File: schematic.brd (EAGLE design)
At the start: 72 x 26 mm, 27 parts, among them IC1 MEGA8-AI

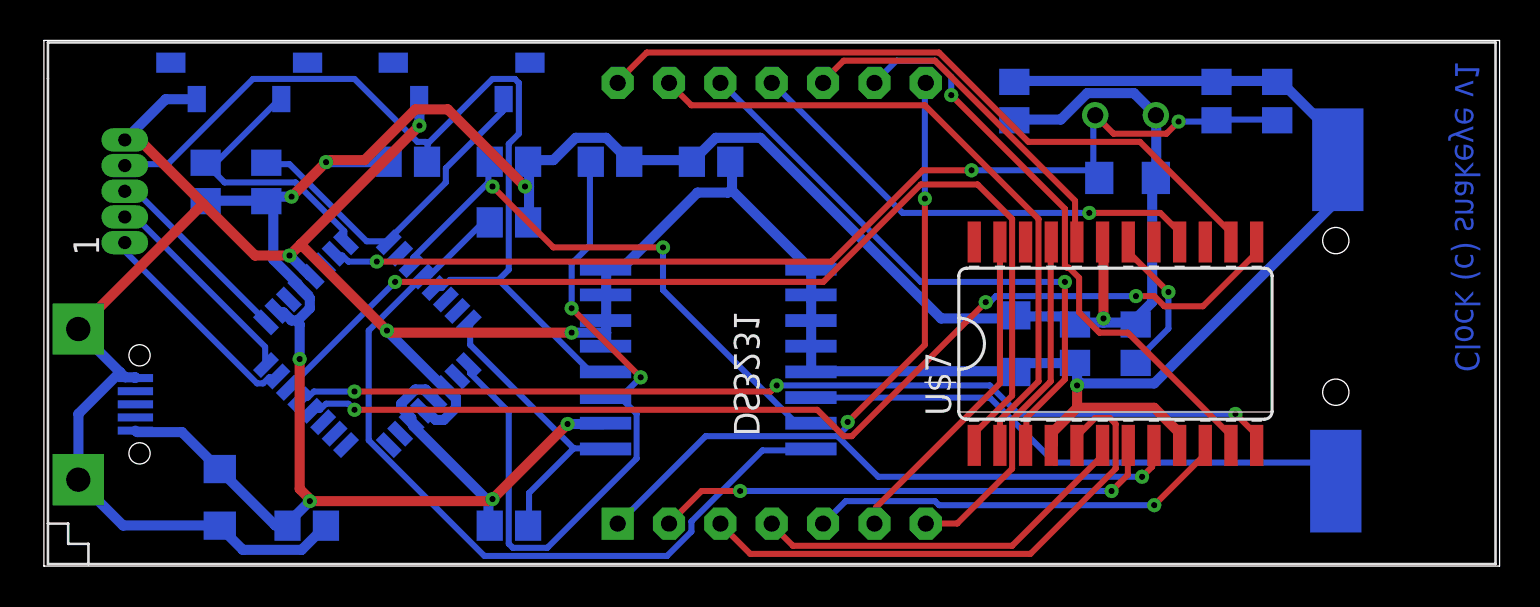
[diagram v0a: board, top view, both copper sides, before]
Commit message: PCB design
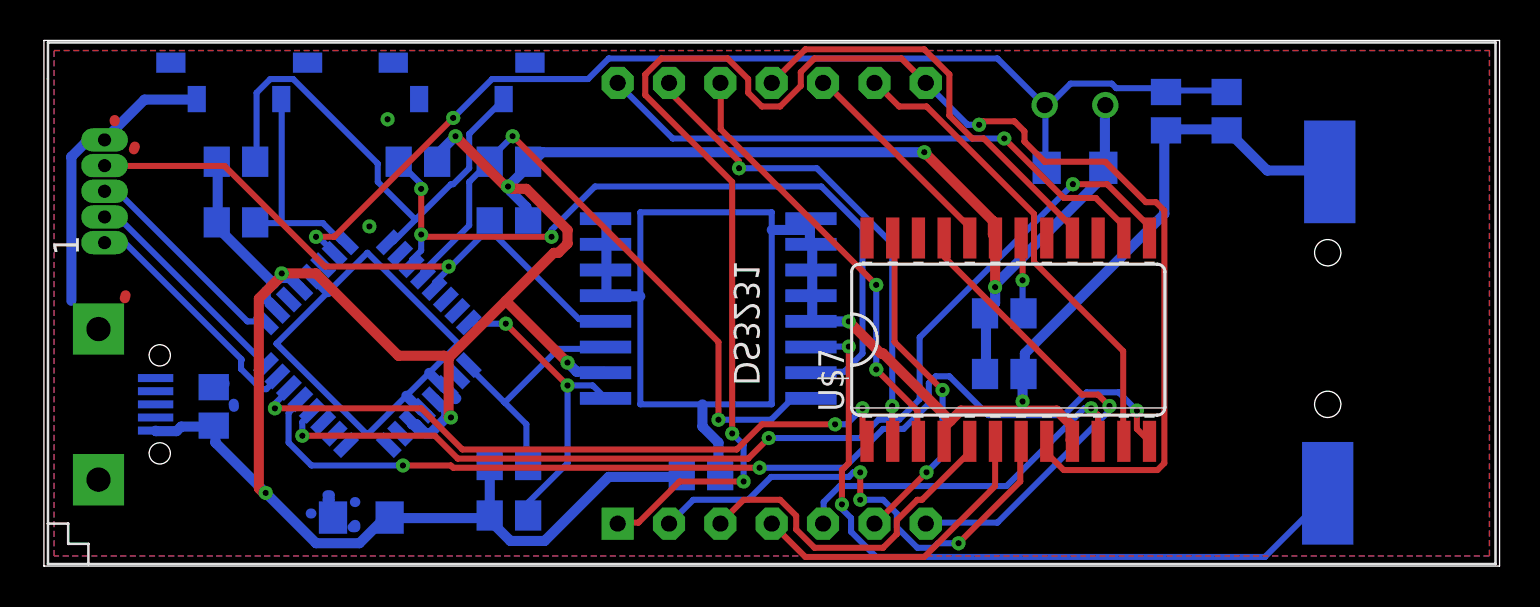
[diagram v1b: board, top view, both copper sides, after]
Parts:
- removed C3: 0.1, resistor:C0805
- removed C7: 10uF, SparkFun-Capacitors:EIA3216
- moved R5 15.8 mm to (23.0, 5.00), turned to 0 degrees
- moved C1 15.5 mm to (32.5, 4.50)
- moved C4 7.48 mm to (8.40, 7.90), turned to 90 degrees
- moved C6 7.07 mm to (15.7, 2.40), turned to 180 degrees
- moved R3 6.67 mm to (47.5, 12.5), turned to 180 degrees
- moved R9 5.83 mm to (23.0, 17.0), turned to 180 degrees
- moved U$7 5.30 mm to (47.7, 11.2)
- moved R1 4.50 mm to (18.5, 20.0)
- moved C2 3.81 mm to (47.5, 9.50), turned to 180 degrees
- moved R2 3.00 mm to (23.0, 20.0)
- moved C8 2.65 mm to (51.0, 19.7)
- moved C5 2.55 mm to (58.5, 22.5), turned to 270 degrees
- moved R7 2.55 mm to (55.5, 22.5), turned to 90 degrees
- moved U$6 2.55 mm to (51.0, 22.8)
- moved R6 2.50 mm to (9.50, 17.0), turned to 0 degrees
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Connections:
- net GND: no longer C3.2, C7.C
- net VCC: no longer C3.1, C7.A
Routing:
- net GND: track 168.9 -> 137.2 mm, vias 5 -> 4
- net N$13: track 49.7 -> 80.9 mm
- net TIMER_INT: track 36.6 -> 12.3 mm, vias 2 -> 0
- net DSP_DIN: track 52.6 -> 33.8 mm, vias 1 -> 3
- net RESET: track 45.6 -> 31.6 mm, vias 0 -> 1
- net SDA: track 28.9 -> 38.9 mm, vias 2 -> 3
- net N$12: track 27.0 -> 17.1 mm
- net N$14: track 27.7 -> 36.8 mm, vias 0 -> 2
- net N$6: track 33.1 -> 24.6 mm, vias 0 -> 2
- net SCL: track 40.4 -> 32.0 mm, vias 0 -> 2
- net N$10: track 30.0 -> 21.8 mm, vias 1 -> 2
- net BTN_2: track 17.1 -> 24.6 mm
- net N$3: track 17.9 -> 10.8 mm
- net DIG_1: track 35.2 -> 28.6 mm, vias 0 -> 1
- net N$5: track 17.4 -> 23.8 mm, vias 0 -> 1
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- added copper zone on layer 1, net GND
- added copper zone on layer 16, net GND
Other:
- board text removed: "Clock (c) snakeye v1"
